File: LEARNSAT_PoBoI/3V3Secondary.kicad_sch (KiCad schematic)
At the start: 17 parts, among them Q1 SI7164DP-T1-GE3, Q4 SI5418DU-T1-GE3, U12 INA219AIDCNR, U15 LTC4231IUD-2#TRPBF

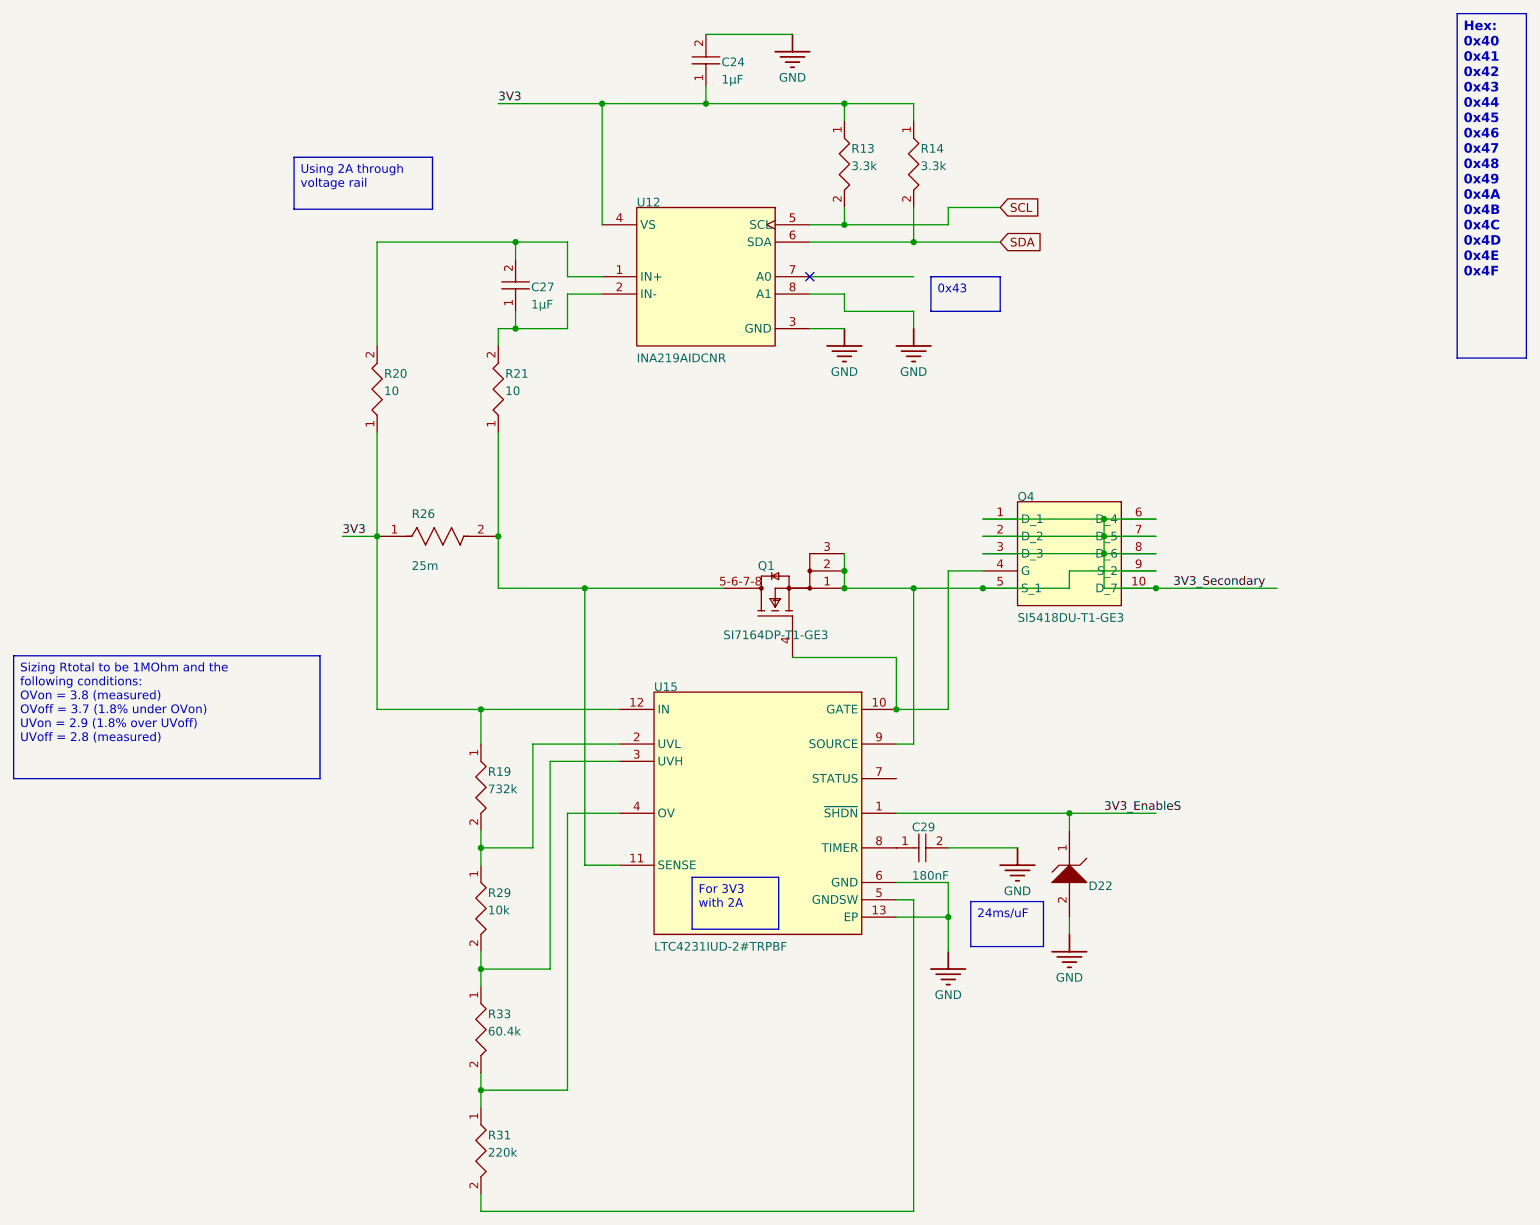
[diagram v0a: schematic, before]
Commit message: Added footprints
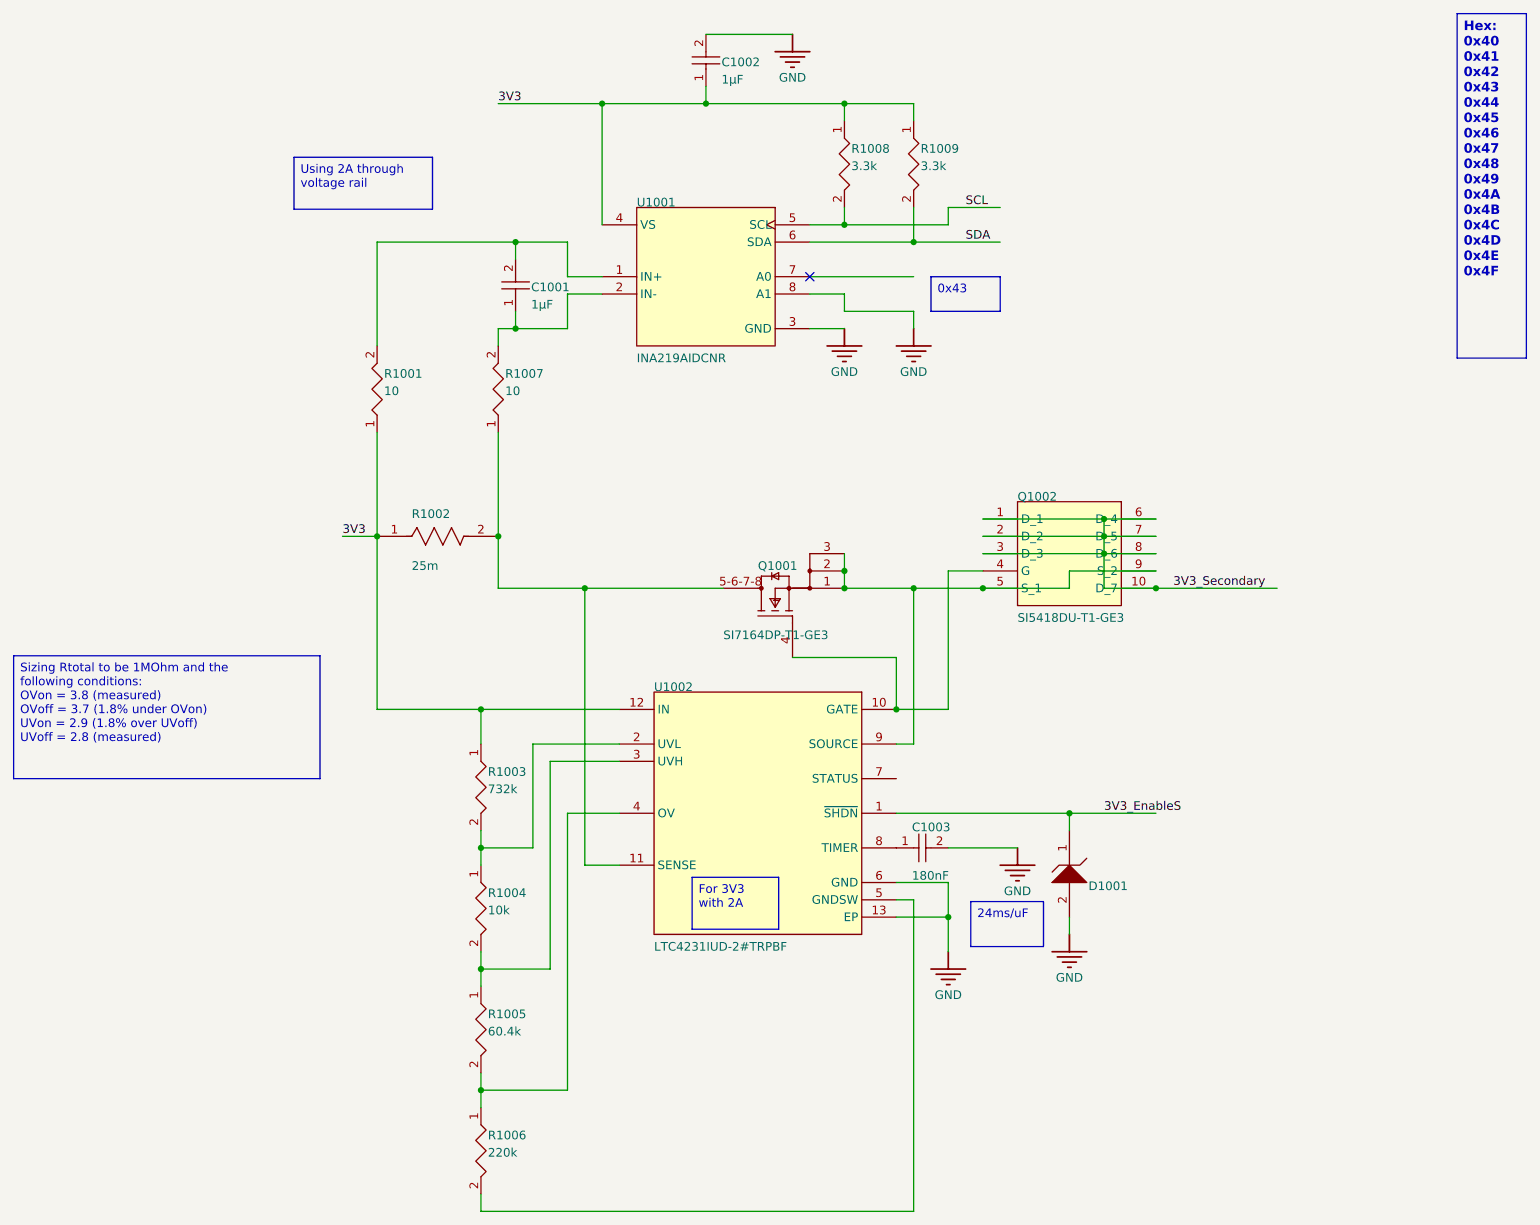
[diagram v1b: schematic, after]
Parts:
- C1001: renamed from C27; footprint CAPC1608X90X40LL10T20 -> Capacitor_SMD:C_0603_1608Metric
- C1002: renamed from C24; footprint CAPC1608X90X35ML15T15 -> Capacitor_SMD:C_0603_1608Metric
- C1003: renamed from C29; footprint FP-C0805C-DN-IPC_A -> Capacitor_SMD:C_0805_2012Metric
- D1001: renamed from D22; footprint ONSC-SOD-323-2-477-02_V -> Diode_SMD:D_SOD-323
- Q1001: renamed from Q1; footprint Vishay_S17-0173-SINGLE_MFG -> Package_SO:Vishay_PowerPAK_1212-8_Single
- Q1002: renamed from Q4; footprint SI5418DU-T1-GE3-Footprint-1 -> Package_SO:Vishay_PowerPAK_1212-8_Single
- R1001: renamed from R20; footprint RESC0402(1005)_L -> Resistor_SMD:R_0402_1005Metric
- R1002: renamed from R26; footprint FP-CSR1206-IPC_C -> Resistor_SMD:R_1206_3216Metric
- R1003: renamed from R19; footprint FP-CR0805-IPC_A -> Resistor_SMD:R_0805_2012Metric
- R1004: renamed from R29; footprint RESC1005X40X25ML05T05 -> Resistor_SMD:R_0402_1005Metric
- R1005: renamed from R33; footprint RESC1005X40X25NL05T10 -> Resistor_SMD:R_0402_1005Metric
- R1006: renamed from R31; footprint FP-ESR01-IPC_C -> Resistor_SMD:R_0402_1005Metric
- R1007: renamed from R21; footprint RESC0402(1005)_L -> Resistor_SMD:R_0402_1005Metric
- R1008: renamed from R13; footprint FP-CRCW1210-e3-IPC_C -> Resistor_SMD:R_1210_3225Metric
- R1009: renamed from R14; footprint FP-CRCW1210-e3-IPC_C -> Resistor_SMD:R_1210_3225Metric
- U1001: renamed from U12; footprint FP-DCN0008A-IPC_A -> INA219AIDCNR:SOT65P280X145-8N
- U1002: renamed from U15; footprint FP-UD-12-05-08-1855-IPC_A -> LTC4231IUD-2_TRPBF:QFN50P300X300X80-13N

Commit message: Add files via upload
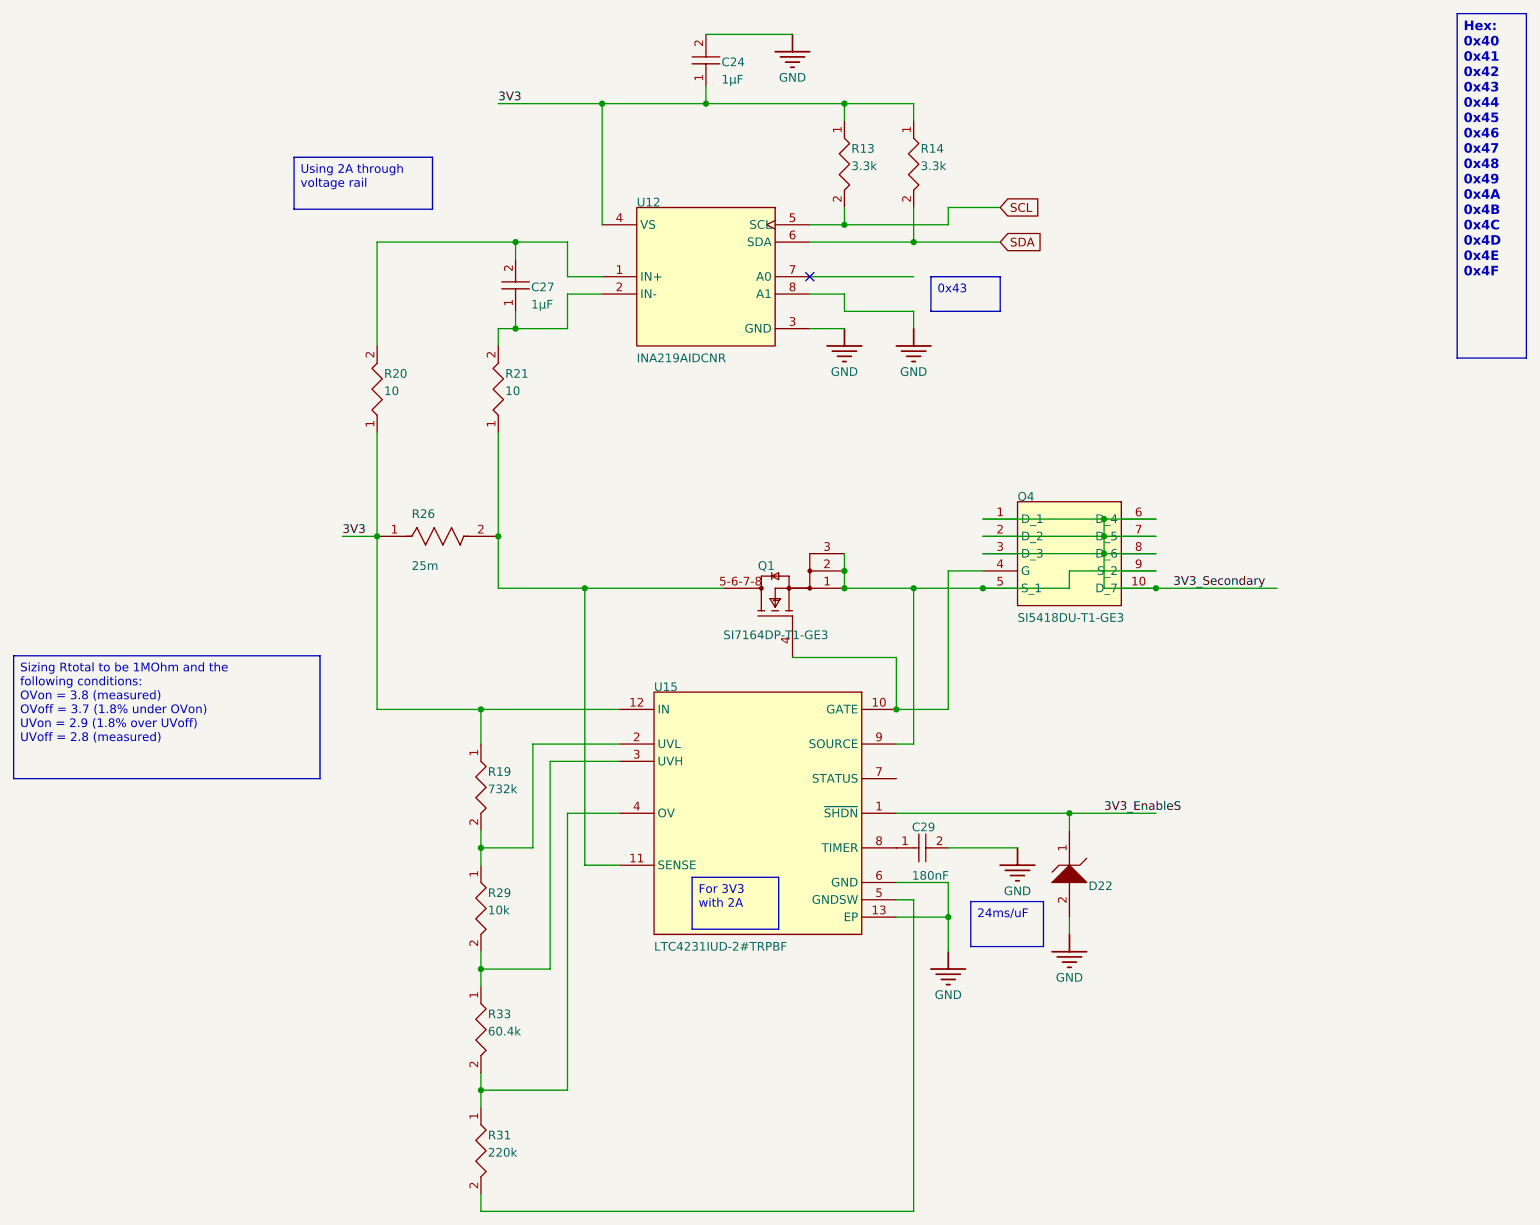
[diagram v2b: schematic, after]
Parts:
- C24: renamed from C1002; footprint Capacitor_SMD:C_0603_1608Metric -> CAPC1608X90X35ML15T15
- C27: renamed from C1001; footprint Capacitor_SMD:C_0603_1608Metric -> CAPC1608X90X40LL10T20
- C29: renamed from C1003; footprint Capacitor_SMD:C_0805_2012Metric -> FP-C0805C-DN-IPC_A
- D22: renamed from D1001; footprint Diode_SMD:D_SOD-323 -> ONSC-SOD-323-2-477-02_V
- Q1: renamed from Q1001; footprint Package_SO:Vishay_PowerPAK_1212-8_Single -> Vishay_S17-0173-SINGLE_MFG
- Q4: renamed from Q1002; footprint Package_SO:Vishay_PowerPAK_1212-8_Single -> SI5418DU-T1-GE3-Footprint-1
- R13: renamed from R1008; footprint Resistor_SMD:R_1210_3225Metric -> FP-CRCW1210-e3-IPC_C
- R14: renamed from R1009; footprint Resistor_SMD:R_1210_3225Metric -> FP-CRCW1210-e3-IPC_C
- R19: renamed from R1003; footprint Resistor_SMD:R_0805_2012Metric -> FP-CR0805-IPC_A
- R20: renamed from R1001; footprint Resistor_SMD:R_0402_1005Metric -> RESC0402(1005)_L
- R21: renamed from R1007; footprint Resistor_SMD:R_0402_1005Metric -> RESC0402(1005)_L
- R26: renamed from R1002; footprint Resistor_SMD:R_1206_3216Metric -> FP-CSR1206-IPC_C
- R29: renamed from R1004; footprint Resistor_SMD:R_0402_1005Metric -> RESC1005X40X25ML05T05
- R31: renamed from R1006; footprint Resistor_SMD:R_0402_1005Metric -> FP-ESR01-IPC_C
- R33: renamed from R1005; footprint Resistor_SMD:R_0402_1005Metric -> RESC1005X40X25NL05T10
- U12: renamed from U1001; footprint INA219AIDCNR:SOT65P280X145-8N -> FP-DCN0008A-IPC_A
- U15: renamed from U1002; footprint LTC4231IUD-2_TRPBF:QFN50P300X300X80-13N -> FP-UD-12-05-08-1855-IPC_A
